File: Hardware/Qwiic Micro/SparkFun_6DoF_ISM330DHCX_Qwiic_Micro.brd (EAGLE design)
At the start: 19.1 x 7.6 mm, 41 parts, among them J1 Qwiic Right Angle, U1 ISM330DHCX

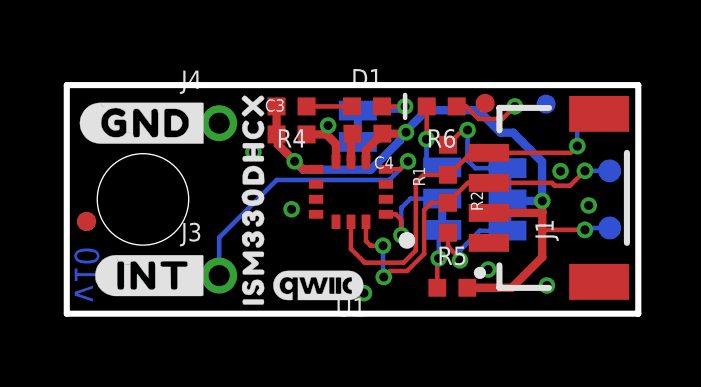
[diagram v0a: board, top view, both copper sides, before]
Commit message: Adds all the measures anyone could want
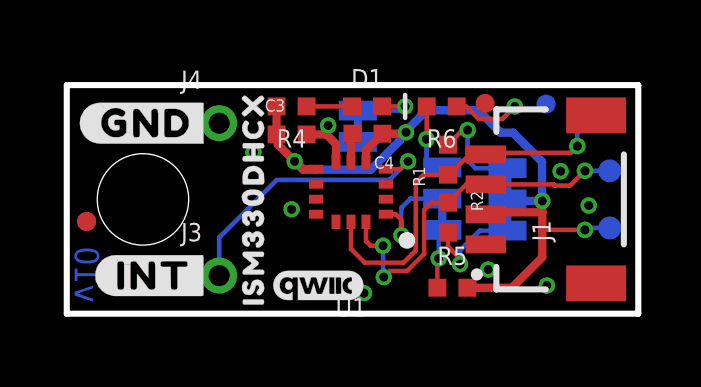
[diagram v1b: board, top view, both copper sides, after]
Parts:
- moved FRAME1 11.7 mm to (-21.6, -22.9)
- moved J1 0.11 mm to (14.0, 3.81)
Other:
- board text added: "Units in Inches"
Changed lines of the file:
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@@
 <layer number="45" name="Holes" color="7" fill="1" visible="yes" active="yes"/>
 <layer number="46" name="Milling" color="3" fill="1" visible="no" active="yes"/>
-<layer number="47" name="Measures" color="7" fill="1" visible="no" active="yes"/>
+<layer number="47" name="Measures" color="7" fill="1" visible="yes" active="yes"/>
 <layer number="48" name="Document" color="7" fill="1" visible="no" active="yes"/>
 <layer number="49" name="Reference" color="13" fill="1" visible="yes" active="yes"/>
@@
 <wire x1="19.05" y1="0" x2="19.05" y2="7.62" width="0.2032" layer="20"/>
 <text x="0.263525" y="0.371475" size="0.8128" layer="16" font="vector" ratio="22" rot="SMR90">v10</text>
-<dimension x1="14.0716" y1="3.8608" x2="13.97" y2="0" x3="22.86" y3="1.9304" textsize="1.778" textratio="15" layer="47" dtype="vertical" unit="inch"/>
 <rectangle x1="9.1948" y1="4.953" x2="9.2456" y2="5.1816" layer="41"/>
-<dimension x1="19.05" y1="8.89" x2="0" y2="8.89" x3="9.525" y3="15.24" textsize="1.778" layer="47" dtype="horizontal" unit="inch"/>
-<dimension x1="2.54" y1="3.81" x2="0" y2="3.81" x3="1.27" y3="11.43" textsize="1.778" layer="47" dtype="horizontal" unit="inch"/>
+<dimension x1="2.54" y1="3.81" x2="0" y2="3.81" x3="1.27" y3="12.7" textsize="1.778" layer="47" dtype="horizontal" unit="inch"/>
 <wire x1="10.541" y1="3.305175" x2="8.636" y2="3.305175" width="0.254" layer="22"/>
 <wire x1="9.144" y1="2.797175" x2="9.144" y2="3.940175" width="0.254" layer="22" curve="180"/>
@@
 <wire x1="8.128" y1="2.921" x2="7.239" y2="3.81" width="0.254" layer="22"/>
 <wire x1="7.366" y1="2.921" x2="8.255" y2="3.81" width="0.254" layer="22"/>
-<dimension x1="0" y1="7.62" x2="0" y2="0" x3="-5.08" y3="3.81" textsize="1.778" layer="47" unit="inch"/>
+<dimension x1="19.05" y1="7.62" x2="0" y2="7.62" x3="9.525" y3="16.51" textsize="1.778" textratio="15" layer="47" unit="inch"/>
+<dimension x1="19.05" y1="0" x2="19.05" y2="7.62" x3="27.94" y3="3.81" textsize="1.778" textratio="15" layer="47" unit="inch"/>
+<dimension x1="2.54" y1="3.81" x2="2.54" y2="0" x3="-10.16" y3="1.905" textsize="1.778" textratio="15" layer="47" unit="inch"/>
+<dimension x1="5.08" y1="1.27" x2="5.08" y2="0" x3="-13.97" y3="0.635" textsize="1.778" textratio="15" layer="47" unit="inch"/>
+<dimension x1="5.08" y1="1.27" x2="0" y2="1.27" x3="2.54" y3="-3.81" textsize="1.778" textratio="15" layer="47" unit="inch"/>
+<dimension x1="5.08" y1="6.35" x2="5.08" y2="1.27" x3="-6.35" y3="3.81" textsize="1.778" textratio="15" layer="47" unit="inch"/>
+<dimension x1="5.08" y1="6.35" x2="19.05" y2="6.35" x3="12.065" y3="10.16" textsize="1.778" textratio="15" layer="47" unit="inch"/>
+<dimension x1="13.97" y1="3.81" x2="13.97" y2="7.62" x3="22.86" y3="5.715" textsize="1.778" textratio="15" layer="47" unit="inch"/>
+<text x="-1.27" y="-10.16" size="1.778" layer="47" font="vector">Units in Inches</text>
 </plain>
 <attributes>
@@
 </autorouter>
 <elements>
-<element name="FRAME1" library="SparkFun-Aesthetics" package="CREATIVE_COMMONS" value="FRAME-LETTER" x="-19.05" y="-11.43" smashed="yes">
-<attribute name="DESIGNER" value="Elias Santistevan" x="12.7" y="-11.43" size="1.778" layer="51" font="vector"/>
-<attribute name="REV" value="" x="-19.05" y="-11.43" size="1.778" layer="27" display="off"/>
+<element name="FRAME1" library="SparkFun-Aesthetics" package="CREATIVE_COMMONS" value="FRAME-LETTER" x="-21.59" y="-22.86" smashed="yes">
+<attribute name="DESIGNER" value="Elias Santistevan" x="10.16" y="-22.86" size="1.778" layer="51" font="vector"/>
+<attribute name="REV" value="" x="-21.59" y="-22.86" size="1.778" layer="27" display="off"/>
 </element>
 <element name="C3" library="SparkFun-Capacitors" package="0402-TIGHT" value="0.1uF" x="7.493" y="5.97535" smashed="yes">
@@
 <attribute name="VALUE" x="12.4968" y="7.6708" size="0.6096" layer="27" font="vector" ratio="20" rot="R180" align="top-center"/>
 </element>
-<element name="J1" library="SparkFun-Connectors" package="JST04_1MM_RA" value="Qwiic Right Angle" x="14.0716" y="3.8608" smashed="yes" rot="R90">
-<attribute name="NAME" x="16.2306" y="2.4638" size="0.6096" layer="25" font="vector" ratio="20" rot="R90"/>
-<attribute name="PROD_ID" value="CONN-13694" x="14.0716" y="3.8608" size="1.778" layer="27" rot="R90" display="off"/>
-<attribute name="VALUE" x="17.3736" y="2.2098" size="0.6096" layer="27" font="vector" ratio="20" rot="R90"/>
+<element name="J1" library="SparkFun-Connectors" package="JST04_1MM_RA" value="Qwiic Right Angle" x="13.97" y="3.81" smashed="yes" rot="R90">
+<attribute name="NAME" x="16.129" y="2.413" size="0.6096" layer="25" font="vector" ratio="20" rot="R90"/>
+<attribute name="PROD_ID" value="CONN-13694" x="13.97" y="3.81" size="1.778" layer="27" rot="R90" display="off"/>
+<attribute name="VALUE" x="17.272" y="2.159" size="0.6096" layer="27" font="vector" ratio="20" rot="R90"/>
 </element>
 <element name="LOGO1" library="SparkFun-Aesthetics" package="QWIIC_3MM" value="QWIIC_LOGO_3MM" x="8.382" y="0.9398" smashed="yes"/>
@@
 <wire x1="9.4742" y1="3.064" x2="9.4742" y2="2.159" width="0.1524" layer="1"/>
 <wire x1="9.9314" y1="1.7018" x2="9.4742" y2="2.159" width="0.1524" layer="1"/>
-<wire x1="14.0716" y1="5.3608" x2="13.47903125" y2="5.3608" width="0.1524" layer="1"/>
-<wire x1="12.70635" y1="4.6308" x2="12.74903125" y2="4.6308" width="0.1524" layer="1"/>
-<wire x1="13.47903125" y1="5.3608" x2="12.74903125" y2="4.6308" width="0.1524" layer="1"/>
+<wire x1="12.74903125" y1="4.6308" x2="12.70635" y2="4.6308" width="0.1524" layer="1"/>
 <wire x1="12.70635" y1="4.6308" x2="11.8952" y2="4.6308" width="0.1524" layer="1"/>
 <wire x1="11.2268" y1="1.7018" x2="9.9314" y2="1.7018" width="0.1524" layer="1"/>
@@
 <wire x1="11.6332" y1="2.1082" x2="11.2268" y2="1.7018" width="0.1524" layer="1"/>
 <contactref element="TP1" pad="1"/>
-<wire x1="14.0716" y1="5.3608" x2="16.7908" y2="5.3608" width="0.1524" layer="1"/>
 <wire x1="16.7908" y1="5.3608" x2="17.018" y2="5.588" width="0.1524" layer="1"/>
 <via x="17.018" y="5.588" extent="1-16" drill="0.3048"/>
@@
 <wire x1="17.2085" y1="6.6675" x2="18.0975" y2="6.6675" width="0.1524" layer="16"/>
 <wire x1="17.018" y1="6.477" x2="17.2085" y2="6.6675" width="0.1524" layer="16"/>
+<wire x1="13.97" y1="5.31" x2="13.42823125" y2="5.31" width="0.1524" layer="1"/>
+<wire x1="13.42823125" y1="5.31" x2="12.74903125" y2="4.6308" width="0.1524" layer="1"/>
+<wire x1="13.97" y1="5.31" x2="14.0208" y2="5.3608" width="0.1524" layer="1"/>
+<wire x1="14.0208" y1="5.3608" x2="16.7908" y2="5.3608" width="0.1524" layer="1"/>
 </signal>
 <signal name="SDA">
@@
 <wire x1="10.541" y1="2.26455" x2="10.13065" y2="2.26455" width="0.1524" layer="1"/>
 <wire x1="10.13065" y1="2.26455" x2="9.9742" y2="2.421" width="0.1524" layer="1"/>
-<wire x1="14.0716" y1="4.3608" x2="13.36675" y2="4.3608" width="0.1524" layer="1"/>
-<wire x1="13.36675" y1="4.3608" x2="12.70635" y2="3.7004" width="0.1524" layer="1"/>
 <wire x1="12.70635" y1="3.7004" x2="12.1586" y2="3.7004" width="0.1524" layer="1"/>
 <via x="10.5664" y="1.2216" extent="1-16" drill="0.3"/>
@@
 <wire x1="17.272" y1="4.7625" x2="18.0975" y2="4.7625" width="0.1524" layer="16"/>
 <via x="17.272" y="4.7625" extent="1-16" drill="0.3048"/>
-<wire x1="16.16909375" y1="4.3608" x2="16.26029375" y2="4.2696" width="0.1524" layer="1"/>
+<wire x1="16.7791" y1="4.2696" x2="17.272" y2="4.7625" width="0.1524" layer="1"/>
+<wire x1="13.97" y1="4.31" x2="16.21989375" y2="4.31" width="0.1524" layer="1"/>
+<wire x1="16.21989375" y1="4.31" x2="16.26029375" y2="4.2696" width="0.1524" layer="1"/>
 <wire x1="16.26029375" y1="4.2696" x2="16.7791" y2="4.2696" width="0.1524" layer="1"/>
-<wire x1="16.7791" y1="4.2696" x2="17.272" y2="4.7625" width="0.1524" layer="1"/>
-<wire x1="14.0716" y1="4.3608" x2="16.16909375" y2="4.3608" width="0.1524" layer="1"/>
+<wire x1="13.97" y1="4.31" x2="13.31595" y2="4.31" width="0.1524" layer="1"/>
+<wire x1="13.31595" y1="4.31" x2="12.70635" y2="3.7004" width="0.1524" layer="1"/>
 </signal>
 <signal name="SA0">
@@
 <wire x1="7.8799" y1="4.814" x2="8.3117" y2="4.814" width="0.2794" layer="1"/>
 <wire x1="7.8799" y1="4.814" x2="7.6139" y2="5.08" width="0.2794" layer="1"/>
-<wire x1="15.8322" y1="3.3608" x2="15.8496" y2="3.3782" width="0.2794" layer="1"/>
-<wire x1="14.0716" y1="3.3608" x2="15.8322" y2="3.3608" width="0.2794" layer="1"/>
 <wire x1="14.464040625" y1="6.033759375" x2="13.716" y2="6.7818" width="0.2794" layer="16"/>
 <wire x1="13.716" y1="6.7818" x2="11.9936" y2="6.7818" width="0.2794" layer="16"/>
@@
 <via x="17.272" y="2.794" extent="1-16" drill="0.3048"/>
 <wire x1="17.272" y1="2.794" x2="15.8496" y2="2.794" width="0.1524" layer="1"/>
+<wire x1="13.97" y1="3.31" x2="14.0382" y2="3.3782" width="0.2794" layer="1"/>
+<wire x1="14.0382" y1="3.3782" x2="15.8496" y2="3.3782" width="0.2794" layer="1"/>
 </signal>
 <signal name="N$5">
@@
 <contactref element="I2C_PU" pad="3"/>
 <contactref element="R2" pad="2"/>
-<via x="13.107228125" y="1.778828125" extent="1-16" drill="0.3"/>
+<via x="13.107228125" y="1.651828125" extent="1-16" drill="0.3"/>
 <wire x1="12.70635" y1="2.7004" x2="12.70635" y2="2.23735625" width="0.1524" layer="1"/>
 <wire x1="13.7668" y1="2.7686" x2="13.107228125" y2="2.109028125" width="0.1524" layer="16"/>
-<wire x1="13.107228125" y1="1.778828125" x2="13.107228125" y2="2.109028125" width="0.1524" layer="16"/>
+<wire x1="13.107228125" y1="1.651828125" x2="13.107228125" y2="2.109028125" width="0.1524" layer="16"/>
 <wire x1="13.7668" y1="2.7686" x2="14.68755" y2="2.7686" width="0.1524" layer="16"/>
-<wire x1="13.107228125" y1="1.836478125" x2="13.107228125" y2="1.778828125" width="0.1524" layer="1"/>
+<wire x1="13.107228125" y1="1.836478125" x2="13.107228125" y2="1.651828125" width="0.1524" layer="1"/>
 <wire x1="12.70635" y1="2.23735625" x2="13.107228125" y2="1.836478125" width="0.1524" layer="1"/>
 </signal>
